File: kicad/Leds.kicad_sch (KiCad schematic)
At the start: 58 parts, among them J20 Conn_01x17, J22 Conn_01x17, J23 Conn_01x17, J24 Conn_01x17, J25 Conn_01x17, J26 Conn_01x17, P10 CONN_8, P4 CONN_8, P5 LEDs, P6 CONN_8, P7 CONN_8, P8 CONN_8, P9 CONN_8, U2 MAX6969, U8 MAX6969, U9 MAX6969

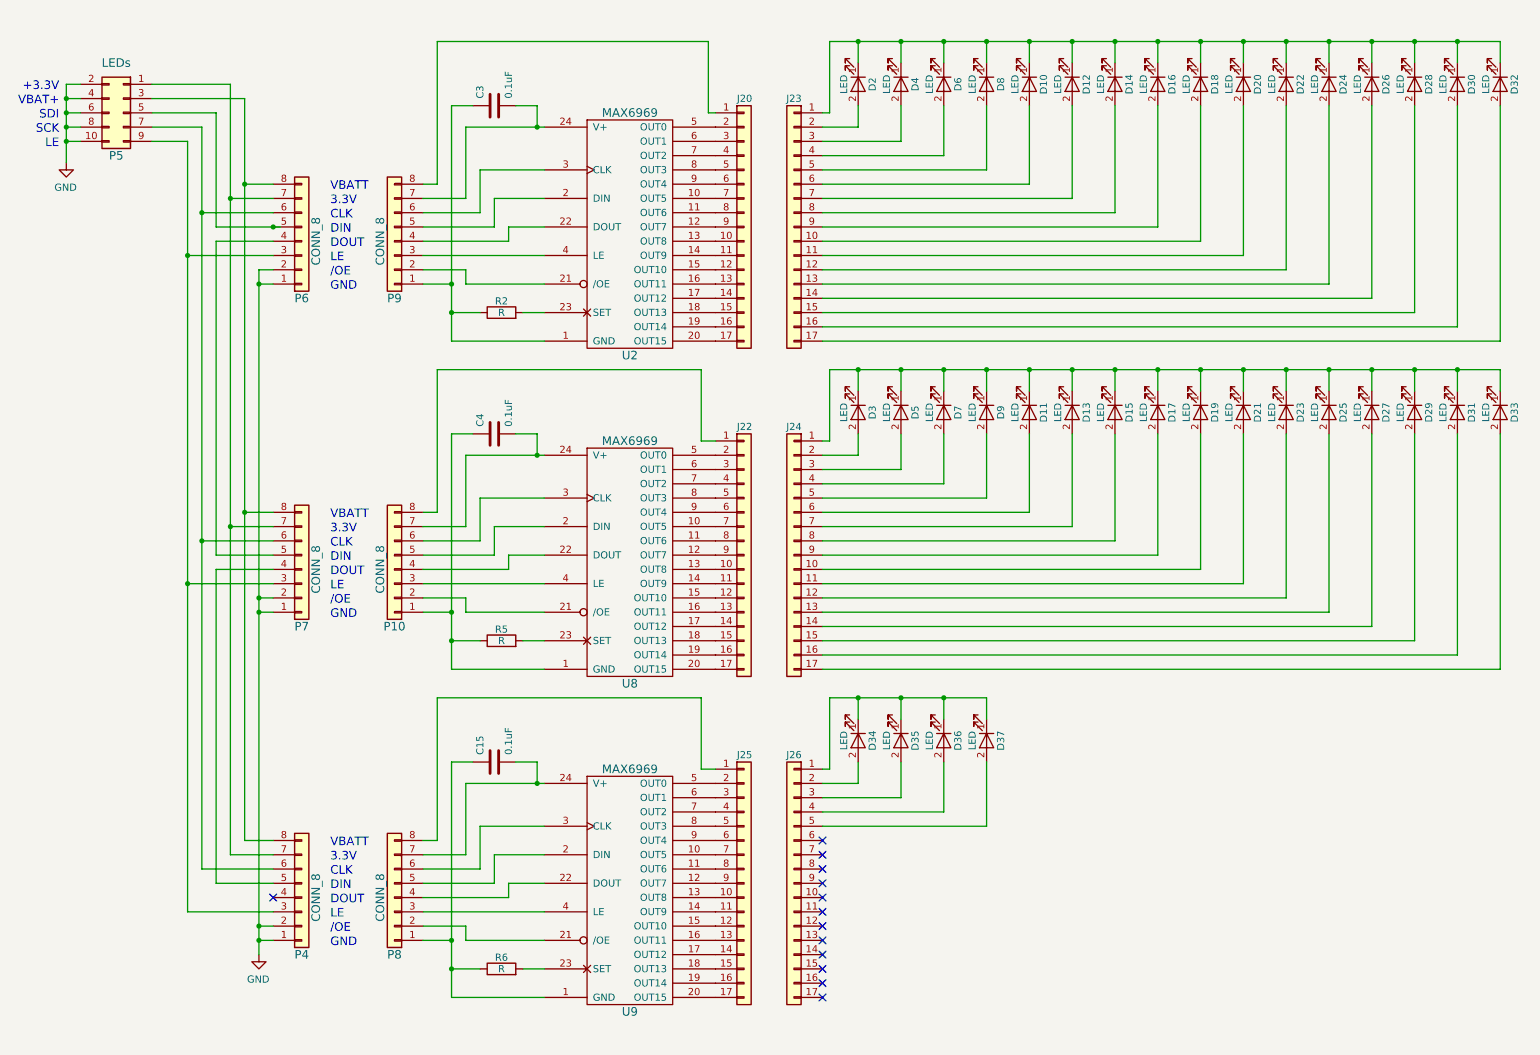
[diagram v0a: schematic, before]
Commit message: Optimizing power lines
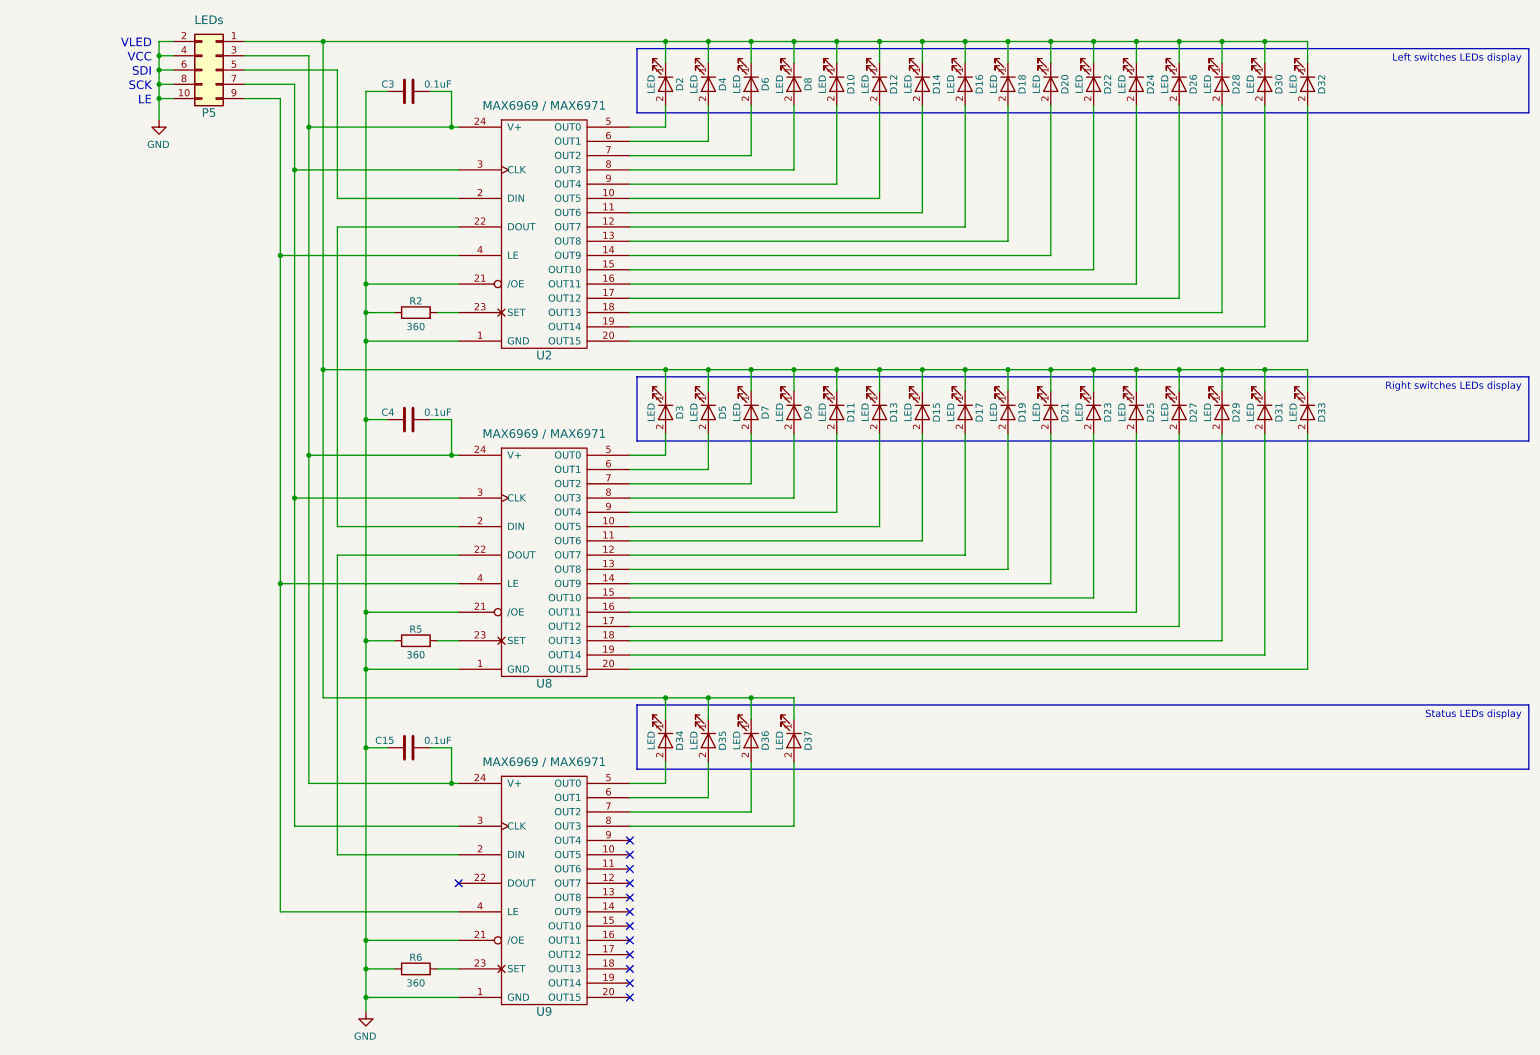
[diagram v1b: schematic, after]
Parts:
- removed J20, J22, J23, J24, J25, J26: Conn_01x17, Connectors_Samtec:SL-117-X-XX_1x17, symbol RCTX-rescue:Conn_01x17-conn
- removed P10, P4, P6, P7, P8, P9: CONN_8, Connectors_Samtec:SL-108-X-XX_1x08, symbol RCTX-rescue:Conn_01x08-conn
- R2, R5, R6: value R -> 360
- U2, U8, U9: value MAX6969 -> MAX6969 / MAX6971
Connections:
- net GND: now also C15.1, C3.1, C4.1, R2.1, R5.1, R6.1, U2.1 (GND), U2.21 (/OE), U8.1 (GND), U8.21 (/OE), U9.1 (GND), U9.21 (/OE)
- net at D10.1 (K), D12.1 (K), D14.1 (K)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: now also D11.1 (K), D13.1 (K), D15.1 (K), D17.1 (K), D19.1 (K), D21.1 (K), D23.1 (K), D25.1 (K), D27.1 (K), D29.1 (K), D3.1 (K), D31.1 (K), D33.1 (K), D34.1 (K), D35.1 (K), D36.1 (K), D37.1 (K), D5.1 (K), D7.1 (K), D9.1 (K), P5.1 (Pin_1)
- net at D30.2 (A): now also U2.19 (OUT14)
- net at C15.2, U9.24 (V+): now also C3.2, C4.2, P5.3 (Pin_3), U2.24 (V+), U8.24 (V+)
- net at D14.2 (A): now also U2.11 (OUT6)
- net at U2.10 (OUT5): now also D12.2 (A)
- net at U2.12 (OUT7): now also D16.2 (A)
- net at U2.13 (OUT8): now also D18.2 (A)
- net at U2.14 (OUT9): now also D20.2 (A)
- net at U2.15 (OUT10): now also D22.2 (A)
- net at U2.16 (OUT11): now also D24.2 (A)
- net at U2.17 (OUT12): now also D26.2 (A)
- net at U2.18 (OUT13): now also D28.2 (A)
- net at U2.2 (DIN): now also P5.5 (Pin_5)
- net at U2.20 (OUT15): now also D32.2 (A)
- net at U2.22 (DOUT): now also U8.2 (DIN)
- net at U2.3 (CLK): now also P5.7 (Pin_7), U8.3 (CLK), U9.3 (CLK)
- net at U2.4 (LE): now also P5.9 (Pin_9), U8.4 (LE), U9.4 (LE)
- net at U2.5 (OUT0): now also D2.2 (A)
- net at U2.6 (OUT1): now also D4.2 (A)
- net at U2.7 (OUT2): now also D6.2 (A)
- net at U2.8 (OUT3): now also D8.2 (A)
- net at U2.9 (OUT4): now also D10.2 (A)
- net at D25.2 (A): now also U8.16 (OUT11)
- net at D23.2 (A): now also U8.15 (OUT10)
- net at D15.2 (A): now also U8.11 (OUT6)
- net at D5.2 (A): now also U8.6 (OUT1)
- net at D33.2 (A): now also U8.20 (OUT15)
- net at D29.2 (A): now also U8.18 (OUT13)
- net at U9.2 (DIN): now also U8.22 (DOUT)
- net at D27.2 (A): now also U8.17 (OUT12)
- net at D3.2 (A): now also U8.5 (OUT0)
- net at D31.2 (A): now also U8.19 (OUT14)
- net at D36.2 (A): now also U9.7 (OUT2)
- net at D19.2 (A): now also U8.13 (OUT8)
- net at D9.2 (A): now also U8.8 (OUT3)
- net at D37.2 (A): now also U9.8 (OUT3)
- net at D7.2 (A): now also U8.7 (OUT2)
- net at U9.5 (OUT0): now also D34.2 (A)
- net at U9.6 (OUT1): now also D35.2 (A)
- net at U8.14 (OUT9): now also D21.2 (A)
- net at U8.9 (OUT4): now also D11.2 (A)
- net at U8.10 (OUT5): now also D13.2 (A)
- net at U8.12 (OUT7): now also D17.2 (A)
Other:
- note added: "Left switches LEDs display"
- note added: "Right switches LEDs display"
- note added: "Status LEDs display"
- note added: "VCC"
- note added: "VLED"
- note removed: "+3.3V"
- note removed: "/OE"
- note removed: "3.3V"
- note removed: "CLK"
- note removed: "DIN"
- note removed: "DOUT"
- note removed: "GND"
- note removed: "VBAT+"
- note removed: "VBATT"
- moved on the sheet: D10, D12, D14, D16, D18, D2, D20, D22, D24, D26, D28, D30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

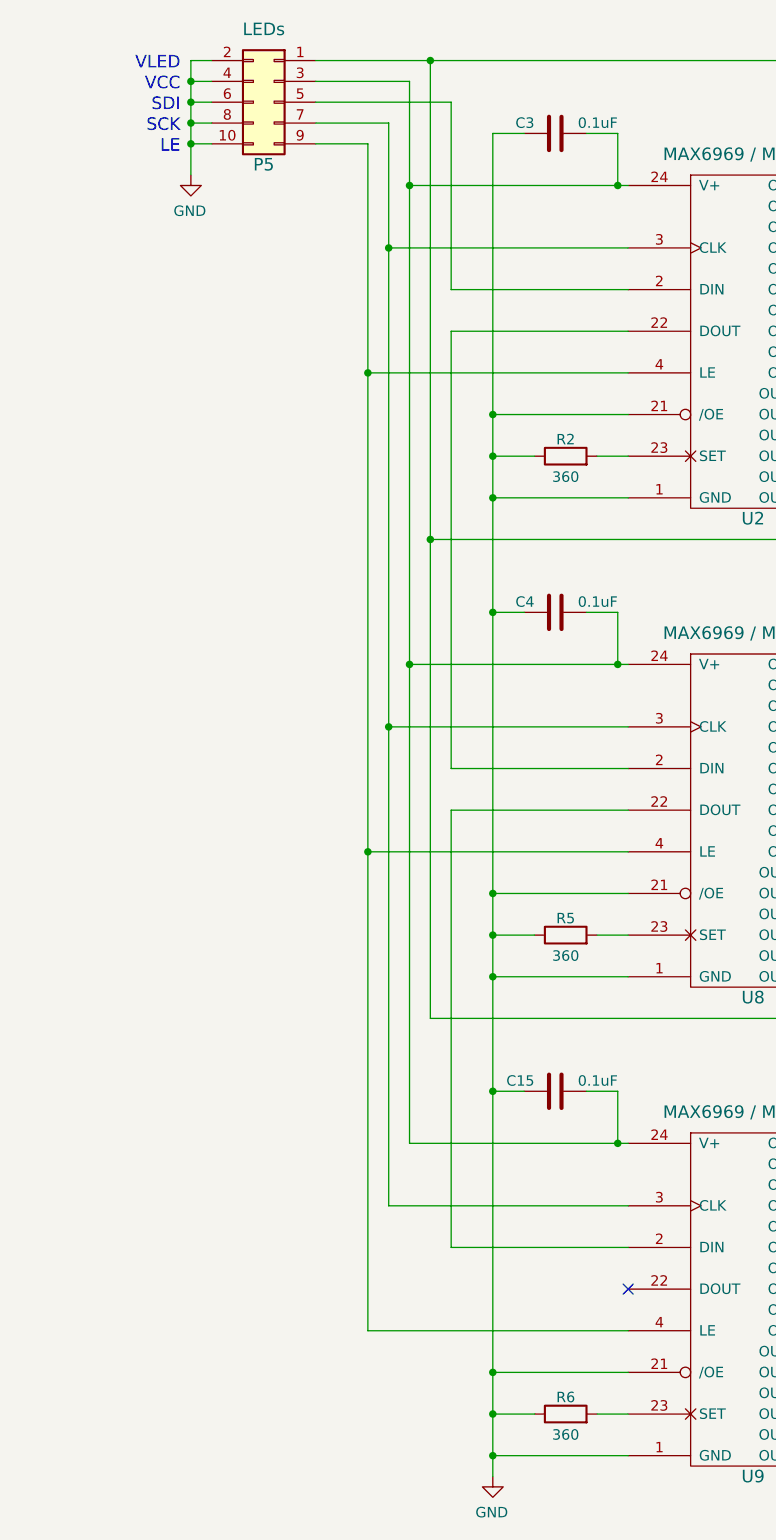
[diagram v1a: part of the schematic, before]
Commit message: Updated the README.md with the preliminary description of the project
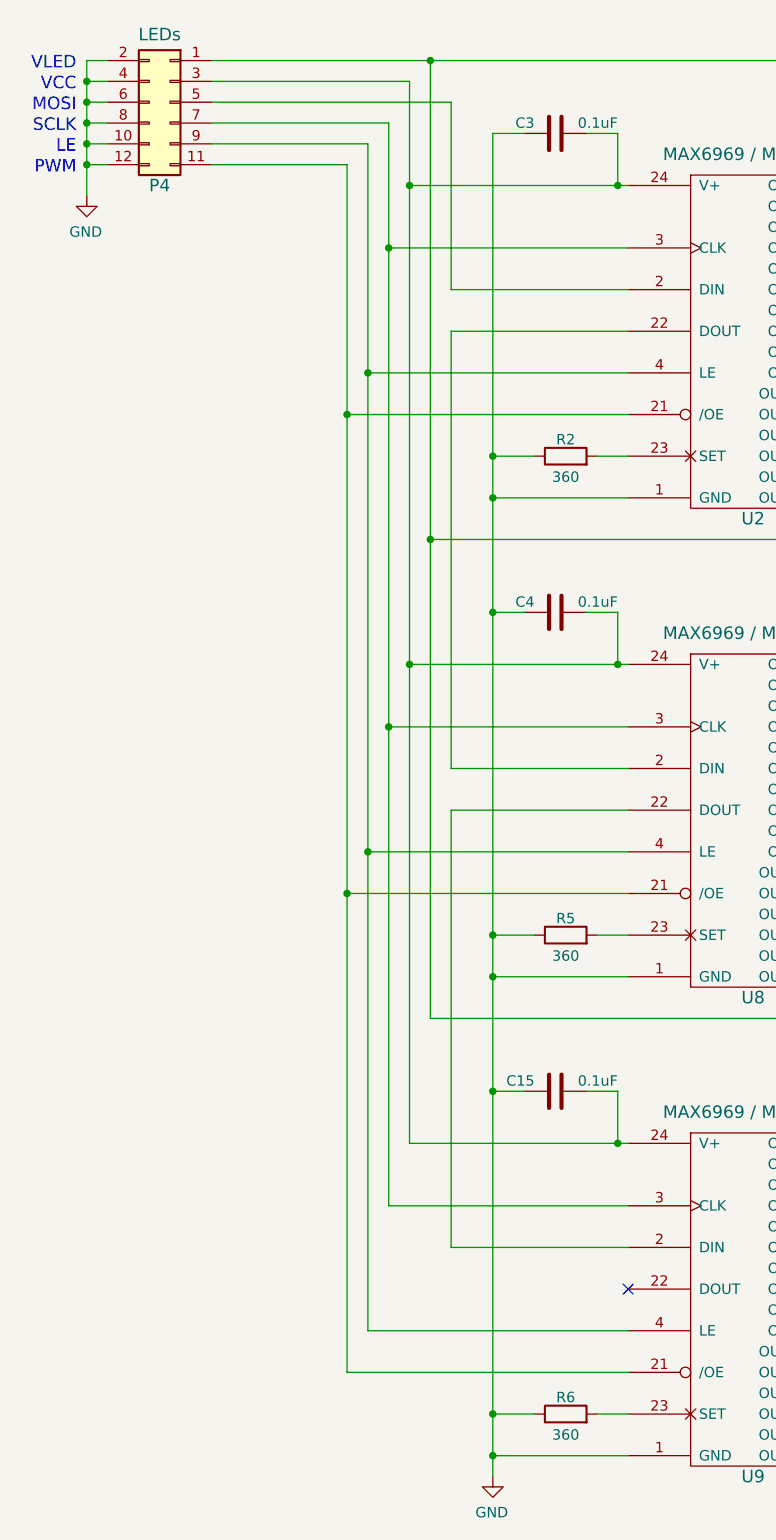
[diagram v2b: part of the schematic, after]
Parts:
- removed P5: LEDs, symbol conn:Conn_02x05_Odd_Even
- added P4: LEDs, symbol conn:Conn_02x06_Odd_Even
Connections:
- net GND: now also P4.10 (Pin_10), P4.12 (Pin_12), P4.2 (Pin_2), P4.4 (Pin_4), P4.6 (Pin_6), P4.8 (Pin_8); no longer U2.21 (/OE), U8.21 (/OE), U9.21 (/OE)
- net at D10.1 (K), D11.1 (K), D12.1 (K)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: now also P4.1 (Pin_1)
- net at U2.2 (DIN): now also P4.5 (Pin_5)
- net at C15.2, C3.2, C4.2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: now also P4.3 (Pin_3)
- net at U2.3 (CLK), U8.3 (CLK), U9.3 (CLK): now also P4.7 (Pin_7)
- net at U2.4 (LE), U8.4 (LE), U9.4 (LE): now also P4.9 (Pin_9)
- new net: P4.11 (Pin_11), U2.21 (/OE), U8.21 (/OE), U9.21 (/OE)
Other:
- note added: "MOSI"
- note added: "PWM"
- note added: "SCLK"
- note removed: "SCK"
- note removed: "SDI"
